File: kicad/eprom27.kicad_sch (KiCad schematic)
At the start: 58 parts, among them P1 POWER_IN, Q1 BSS84LT1, Q2 BSS84LT1, Q3 BC847, Q4 BC847, Q5 BC847, Q6 BSS84LT1, Q7 BSS84LT1, Q8 BSS84LT1, U1 74HC595, U2 74HC595, U3 MT3608, U4 ZIF28

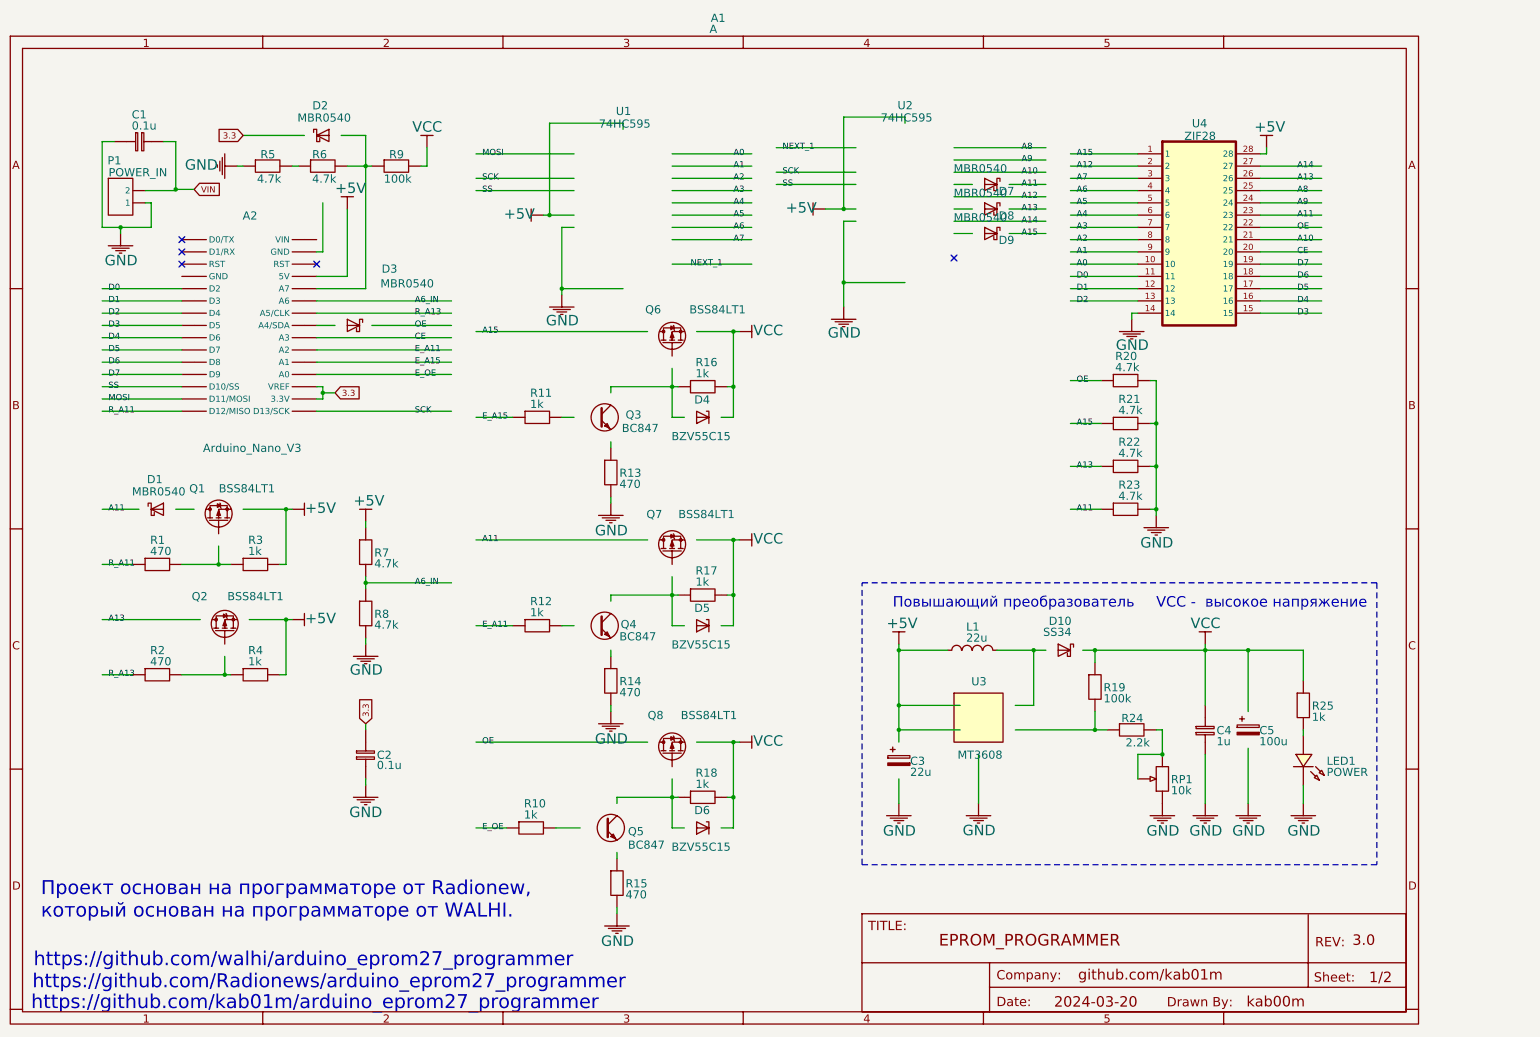
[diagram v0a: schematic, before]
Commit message: Small pre-release fixes
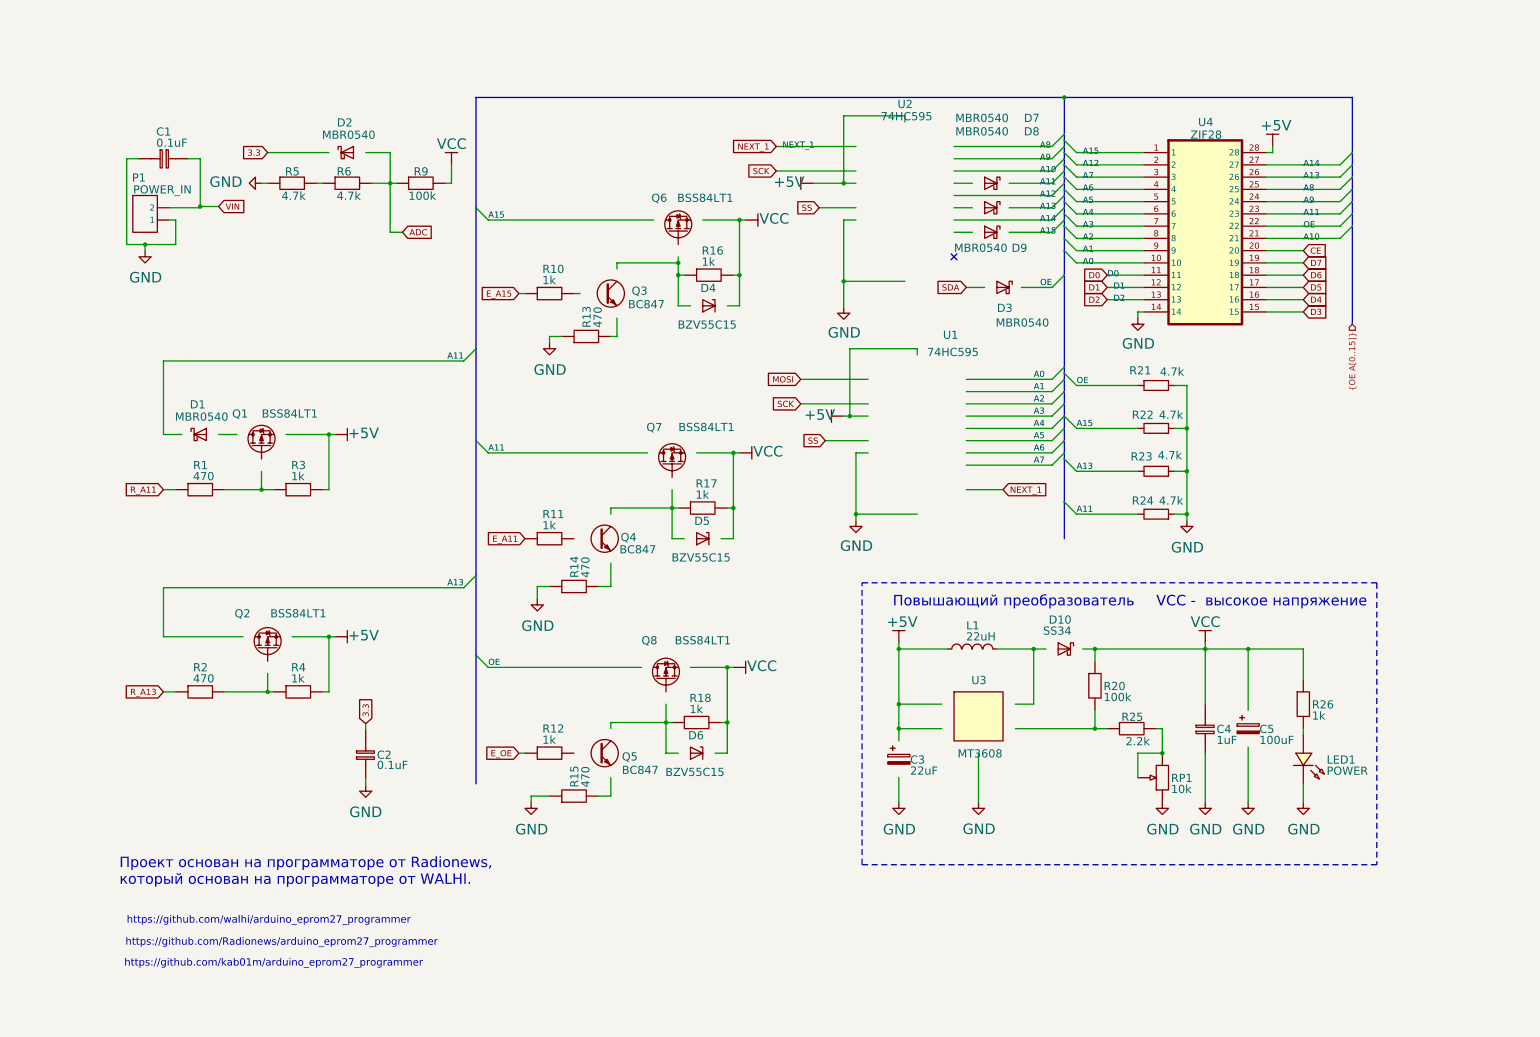
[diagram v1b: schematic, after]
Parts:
- removed A1: A, symbol Unknown_20_-821
- removed A2: Arduino_Nano_V3, symbol Arduino_Nano_V3
- removed R7: 4.7k, Resistor_SMD:R_0805_2012Metric_Pad1.20x1.40mm_HandSolder, symbol R_AXIAL-0.3_EU_1
- removed R8: 4.7k, Resistor_SMD:R_0805_2012Metric_Pad1.20x1.40mm_HandSolder, symbol R_AXIAL-0.3_EU
- C1, C2: value 0.1u -> 0.1uF
- C3: value 22u -> 22uF
- C4: value 1u -> 1uF
- C5: value 100u -> 100uF
- L1: value 22u -> 22uH
- R21: renamed from R20; symbol R_0805_EU_8 -> Device:R
- R22: renamed from R21; symbol R_0805_EU_7 -> Device:R
- R23: renamed from R22; symbol R_0805_EU_6 -> Device:R
- R24: renamed from R23; symbol R_0805_EU_5 -> Device:R
- renumbered R11 to R10, R12 to R11, R10 to R12, R19 to R20, R24 to R25, R25 to R26
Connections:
- net ADC: now reaches R6.2, R9.1
- removed net GND: C1.2, C2.1, C4.1, LED1.2, P1.1, R13.1, R14.1, R15.1, R21.1, R22.2, R23.2, R24.2, R5.1, RP1.1, U4.14
- new net: R21.1, R22.2, R23.2, R24.2
- new net: C1.2, P1.1
- no-connect marks 5 -> 1
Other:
- note added: "Проект основан на программаторе от Radionews, который основан на программаторе от WALHI."
- note removed: "Проект основан на программаторе от Radionew, который основан на программаторе от WALHI."
- company: (none) -> kab01m@github
- title: (none) -> EPROM27 Arduino programmer
- moved on the sheet: C1, D1, D2, D3, D4, D5, D6, P1, Q1, Q2, Q3, Q4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
